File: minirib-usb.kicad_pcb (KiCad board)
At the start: 2 copper layers, 49.5 x 22.5 mm, 48 parts, among them J1 USB_B_Mini, J2 Mini-DIN-6-Shielded, Q1 MMST3904-7-F, Q2 MMST3906-7-F, Q3 MMST3906-7-F, Q4 MMST3904-7-F, Q5 MMST3904-7-F, Q6 MMST3904-7-F, Q7 MMST3904-7-F, U1 FT231XS, U2 TL081H

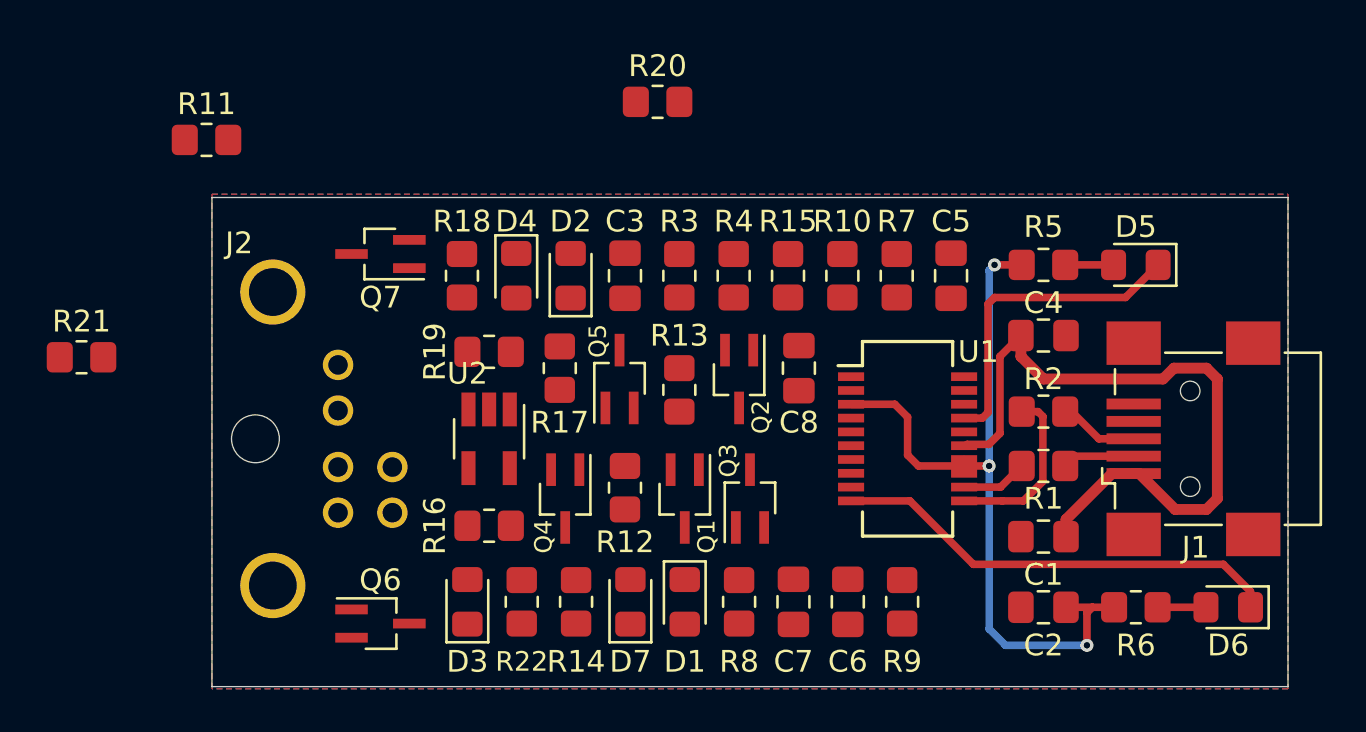
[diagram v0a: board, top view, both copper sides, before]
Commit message: Finalized rev A schematic and PCB
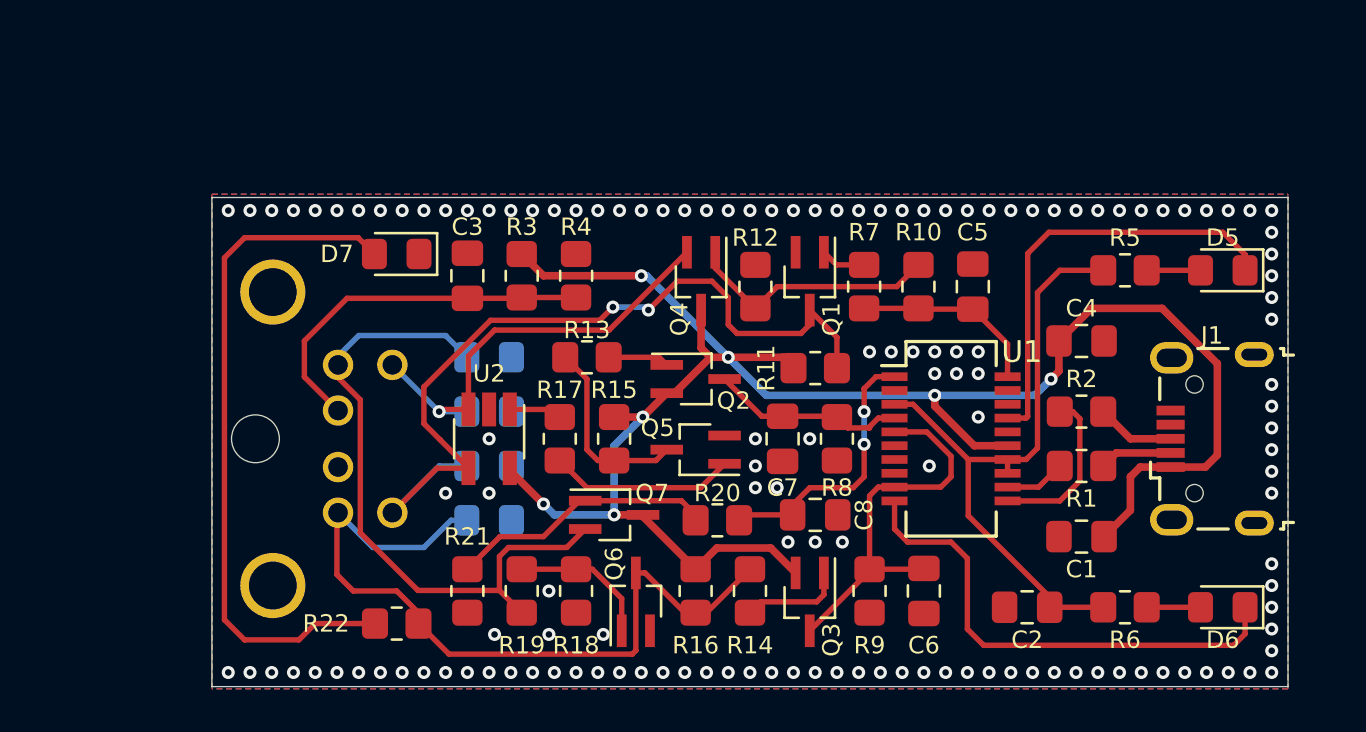
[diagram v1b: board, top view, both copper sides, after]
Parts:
- added G***: LOGO, w3axl-logos:logo-4.2x4.2, B.Cu at (167.2, 107.5)
- D1, D2, D3, D4: moved to B.Cu
- J1: value USB_B_Mini -> USB_B_Micro; footprint Connector_USB:USB_Mini-B_Wuerth_65100516121_Horizontal -> Connector_USB:USB_Micro-B_Wuerth_629105150521
- J2: footprint MiniRIB-USB:MDJ-006-FS -> MiniRIB-USB:KMDGX-6S-BS
- moved R11 29.9 mm to (150.2, 96.8), turned to 180 degrees
- moved R21 20.8 mm to (134.2, 107.0), turned to 90 degrees
- moved R20 19.4 mm to (145.8, 103.8)
- moved D7 19.3 mm to (131.0, 91.5), turned to 180 degrees
- moved Q7 16.1 mm to (141.0, 103.5), turned to 0 degrees
- moved R18 15.4 mm to (139.2, 107.0), turned to 90 degrees
- moved D1 12.6 mm to (135.2, 98.8), turned to 0 degrees
- moved Q6 11.8 mm to (142.0, 107.5), turned to 90 degrees
- moved Q4 11.8 mm to (145.0, 92.8)
- moved Q1 11.5 mm to (150.0, 92.8)
- moved R19 11.1 mm to (136.8, 107.0), turned to 90 degrees
- moved R12 11.0 mm to (147.5, 93.0), turned to 270 degrees
- moved R15 11.0 mm to (141.0, 100.0)
- moved R16 9.96 mm to (144.8, 107.0), turned to 90 degrees
- moved D4 8.84 mm to (135.2, 101.2), turned to 180 degrees
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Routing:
- net +5V: track 32.6 -> 87.7 mm, vias 0 -> 7
- net BUS+: track 0.00 -> 39.1 mm, vias 0 -> 2
- net BUSY: track 0.00 -> 36.0 mm
- net Net-(D7-Pad2): track 0.00 -> 31.9 mm
- net ~BUSY: track 0.00 -> 30.3 mm
- net BUS-: track 0.00 -> 20.2 mm, vias 0 -> 1
- net ~CTS: track 0.00 -> 18.0 mm
- net BIAS: track 0.00 -> 17.2 mm
- net Net-(Q7-Pad1): track 0.00 -> 12.8 mm
- net ~DTR: track 0.00 -> 12.4 mm, vias 0 -> 2
- net Net-(Q4-Pad1): track 0.00 -> 11.7 mm
- net RXD: track 0.00 -> 9.04 mm
- net TXD: track 0.00 -> 8.78 mm
- net Net-(Q5-Pad3): track 0.00 -> 8.75 mm
- net Net-(Q5-Pad1): track 0.00 -> 8.55 mm
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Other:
- board text added: "MiniRIB USB rev A - 2021/12/9"
